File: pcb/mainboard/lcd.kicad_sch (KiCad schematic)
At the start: 18 parts, among them J501 Conn_02x15_Odd_Even_MountingP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, U201 MIMX8MN6DVTJZAA, U502 TPS65632

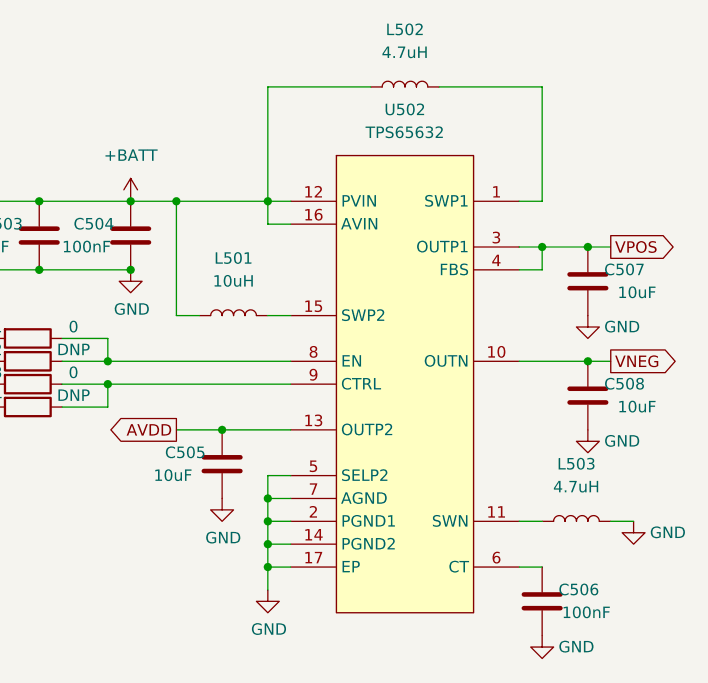
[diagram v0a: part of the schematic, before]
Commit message: Keypad bugfix, pulling in submodules
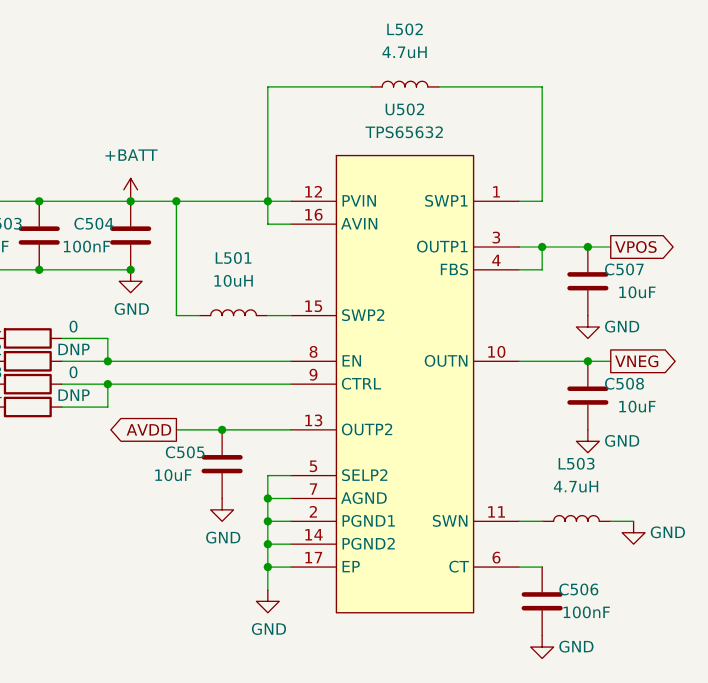
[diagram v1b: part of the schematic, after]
